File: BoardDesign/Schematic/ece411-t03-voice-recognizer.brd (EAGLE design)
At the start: 92.7 x 63.5 mm, 52 parts, among them J1 5.5x2.1mm Barrel, Q1 16MHz, X1 USB-A

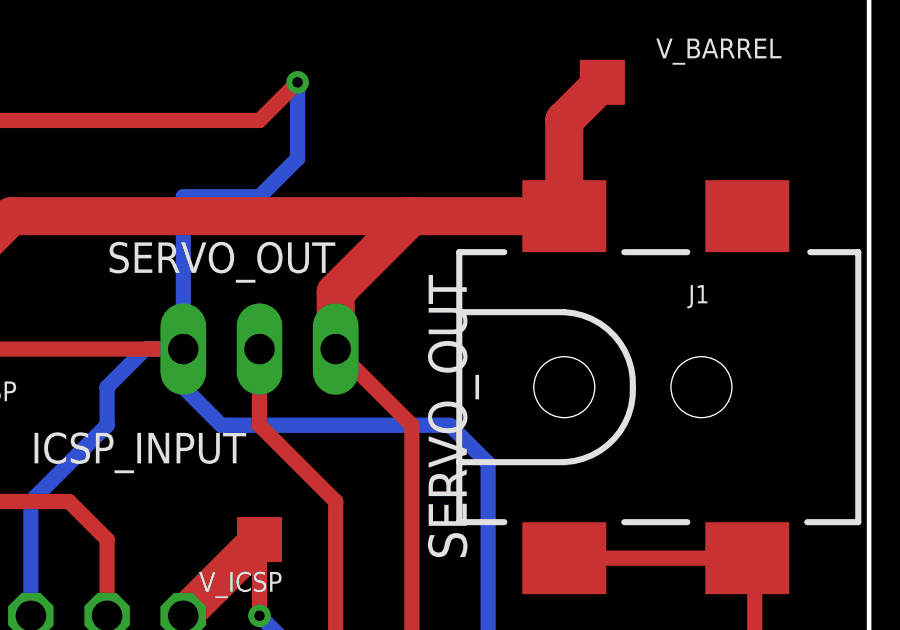
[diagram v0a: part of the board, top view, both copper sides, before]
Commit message: asdf
asdasfsadfsfd
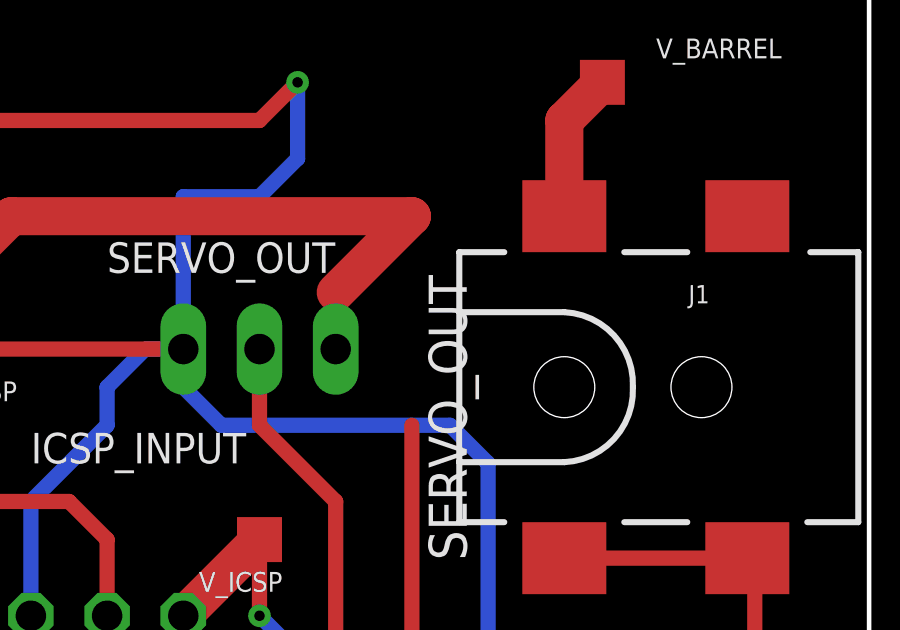
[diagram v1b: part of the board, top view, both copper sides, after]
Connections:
- net N$7: now also J1.VIN0, SERVO_OUT.1, V_BARREL.TP; no longer TP_USB.TP, X1.1
- net VCC: now also TP_USB.TP, X1.1; no longer J1.VIN0, SERVO_OUT.1, V_BARREL.TP
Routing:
- net VCC: track 295.6 -> 287.8 mm
- net N$7: track 7.74 -> 4.99 mm
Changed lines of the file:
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@@
 <wire x1="53.34" y1="29.87" x2="56.43" y2="29.87" width="0.508" layer="1"/>
 <wire x1="85.09" y1="44.45" x2="82.55" y2="41.91" width="1.27" layer="1"/>
-<contactref element="J1" pad="VIN0"/>
-<contactref element="SERVO_OUT" pad="1"/>
-<contactref element="V_BARREL" pad="TP"/>
 <wire x1="63.5" y1="7.62" x2="63.5" y2="2.54" width="1.27" layer="1"/>
 <wire x1="68.03" y1="23.47" x2="65.43" y2="23.47" width="0.508" layer="1"/>
-<wire x1="95.25" y1="55.23" x2="90.17" y2="55.23" width="1.27" layer="1"/>
-<wire x1="95.25" y1="58.42" x2="96.52" y2="59.69" width="1.27" layer="1"/>
-<wire x1="95.25" y1="58.42" x2="95.25" y2="55.23" width="1.27" layer="1"/>
 <wire x1="90.17" y1="55.23" x2="87.63" y2="52.69" width="1.27" layer="1"/>
-<wire x1="87.63" y1="52.69" x2="87.63" y2="50.8" width="1.27" layer="1"/>
 <contactref element="C9" pad="1"/>
 <contactref element="U$1" pad="44"/>
@@
 <wire x1="35.69" y1="36.83" x2="35.69" y2="52.2" width="1.27" layer="1"/>
 <wire x1="35.69" y1="52.2" x2="38.1" y2="54.61" width="1.27" layer="1"/>
-<wire x1="90.17" y1="48.26" x2="87.63" y2="50.8" width="0.508" layer="1"/>
 <wire x1="54.74" y1="11.43" x2="54.61" y2="11.56" width="0.508" layer="1"/>
 <wire x1="54.74" y1="11.43" x2="57.15" y2="11.43" width="0.508" layer="1"/>
@@
 <via x="90.17" y="39.37" extent="1-16" drill="0.35"/>
 <wire x1="90.17" y1="39.37" x2="90.17" y2="48.26" width="0.508" layer="1"/>
+<contactref element="X1" pad="1"/>
+<contactref element="TP_USB" pad="TP"/>
+<wire x1="90.17" y1="22.86" x2="87.57" y2="20.26" width="0.508" layer="1"/>
+<wire x1="87.57" y1="16.2" x2="87.57" y2="20.26" width="0.508" layer="1"/>
+<wire x1="87.63" y1="52.69" x2="90.17" y2="48.26" width="0" layer="19" extent="1-1"/>
+<wire x1="90.17" y1="22.86" x2="90.17" y2="39.37" width="0" layer="19" extent="1-1"/>
 </signal>
 <signal name="SIGNAL">
@@
 <wire x1="67.31" y1="33.55" x2="67.31" y2="35.56" width="0.508" layer="1"/>
 <wire x1="67.31" y1="35.56" x2="69.85" y2="38.1" width="0.508" layer="1"/>
-</signal>
-<signal name="N$7">
-<contactref element="X1" pad="1"/>
-<contactref element="TP_USB" pad="TP"/>
-<wire x1="90.17" y1="22.86" x2="87.57" y2="20.26" width="0.508" layer="1"/>
-<wire x1="87.57" y1="16.2" x2="87.57" y2="20.26" width="0.508" layer="1"/>
 </signal>
 <signal name="MISO">
@@
 <wire x1="38.1" y1="29.21" x2="35.69" y2="31.75" width="0.508" layer="1"/>
 </signal>
+<signal name="N$7">
+<contactref element="J1" pad="VIN0"/>
+<contactref element="SERVO_OUT" pad="1"/>
+<contactref element="V_BARREL" pad="TP"/>
+<wire x1="95.25" y1="58.42" x2="96.52" y2="59.69" width="1.27" layer="1"/>
+<wire x1="95.25" y1="58.42" x2="95.25" y2="55.23" width="1.27" layer="1"/>
+<wire x1="87.63" y1="50.8" x2="95.25" y2="55.23" width="0" layer="19" extent="1-1"/>
+</signal>
 </signals>
